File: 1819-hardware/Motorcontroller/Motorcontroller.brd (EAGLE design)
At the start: 44.8 x 54 mm, 36 parts, among them U1 MAX3485CSA, U3 PCA9306, U4 74HC1G04

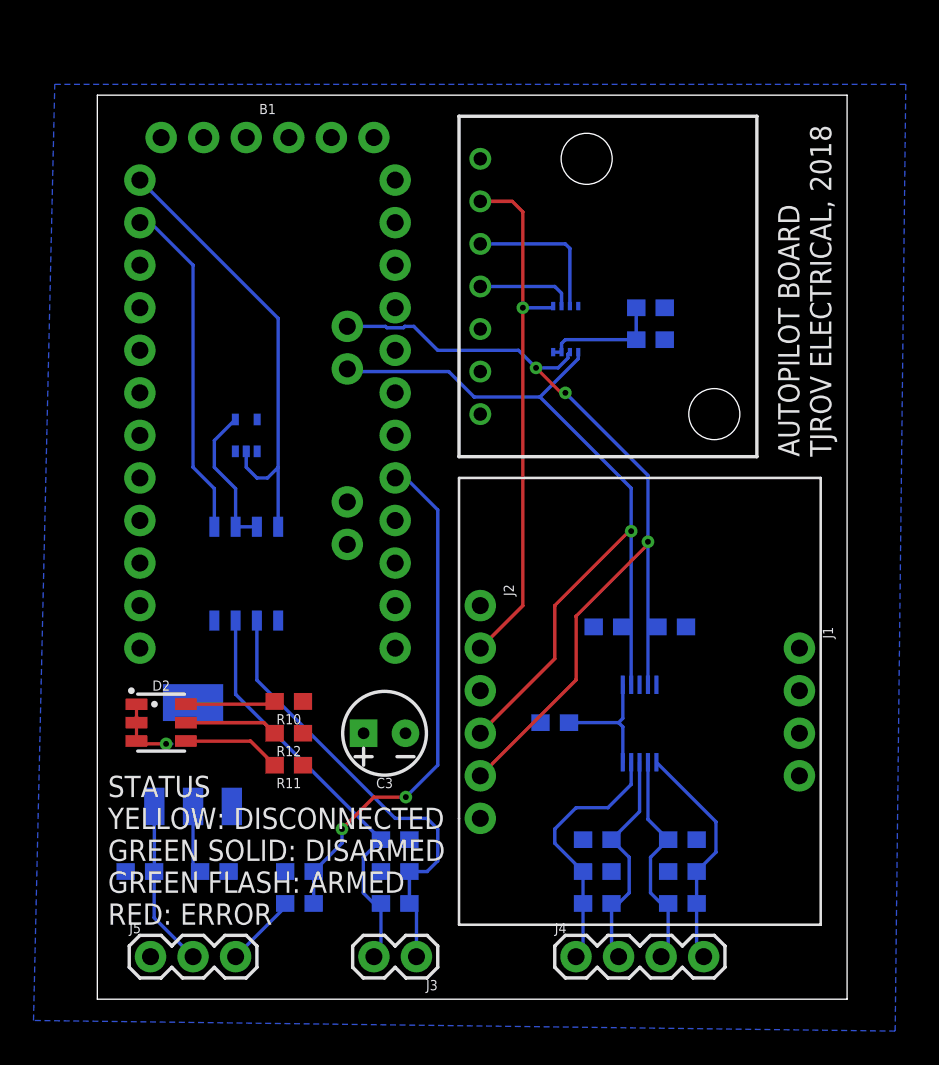
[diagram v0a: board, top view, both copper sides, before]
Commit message: started motorcontroller board files
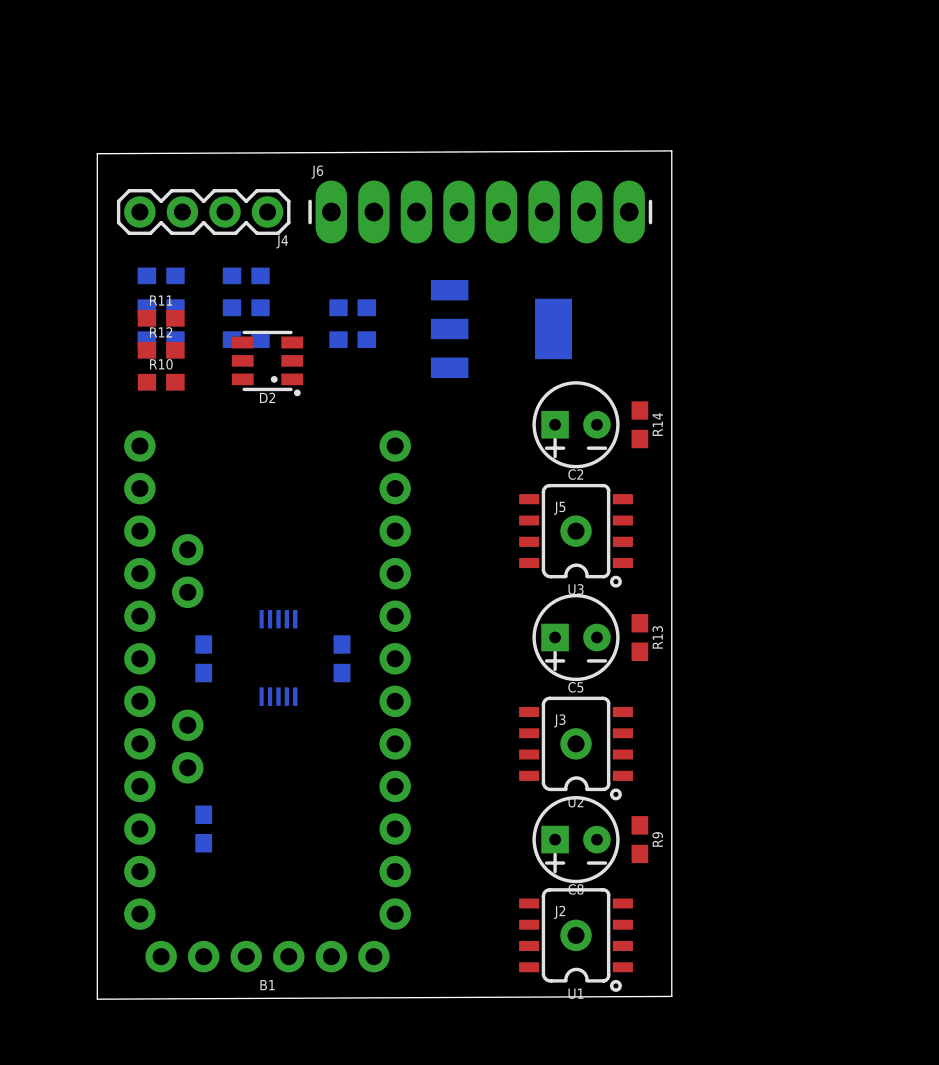
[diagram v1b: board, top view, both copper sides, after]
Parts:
- removed B2: Pressure Sensor, SparkFun-Boards:SPARKFUN_MS5803-14BA_BREAKOUT
- removed J1: (no value), SparkFun-Connectors:1X04_NO_SILK
- removed R15, R17: 4.7k, SparkFun-Resistors:0603
- removed R16: 100k, SparkFun-Resistors:0603
- removed U4: 74HC1G04, SparkFun-IC-Logic:SOT353
- added C8: 10uF, SparkFun-Capacitors:CPOL-RADIAL-2.5MM-5MM
- added J6: (no value), SparkFun-Connectors:1X08_LONGPADS
- added U2: GENERIC-SOIC8MSGEQ7N-FILTER, SparkFun-Retired:SO08
- C2, C5: value 0.1uF -> 10uF; device SparkFun-Capacitors:0603 -> SparkFun-Capacitors:CPOL-RADIAL-2.5MM-5MM
- C3: value 10uF -> 0.1uF; device SparkFun-Capacitors:CPOL-RADIAL-2.5MM-5MM -> SparkFun-Capacitors:0603
- J2: device SparkFun-Connectors:1X06_NO_SILK -> SparkFun-Connectors:1X01_NO_SILK
- J3: device SparkFun-Connectors:1X02 -> SparkFun-Connectors:1X01_NO_SILK
- J5: device SparkFun-Connectors:1X03 -> SparkFun-Connectors:1X01_NO_SILK
- R1: value 100 -> 4.7k
- R13: value 100k -> 47k
- R14: value 4.7k -> 47k
- R4: value 680 -> 4.7k
- R9: value 680 -> 47k
- U1: value MAX3485CSA -> GENERIC-SOIC8MSGEQ7N-FILTER; device SparkFun-IC-Comms:SO08 -> SparkFun-Retired:SO08
- U3: value PCA9306 -> GENERIC-SOIC8MSGEQ7N-FILTER; device SparkFun-IC-Comms:PSOP-8 -> SparkFun-Retired:SO08
- moved FRAME1 121.6 mm to (-80.0, 47.0)
- moved R3 48.7 mm to (3.81, 43.2), turned to 180 degrees
- moved J4 48.1 mm to (10.2, 47.0), turned to 180 degrees
- moved R6 45.8 mm to (3.81, 41.3), turned to 0 degrees
- moved R7 43.1 mm to (3.81, 39.4), turned to 0 degrees
- moved R2 42.9 mm to (8.89, 43.2), turned to 0 degrees
- moved R5 39.6 mm to (8.89, 41.3), turned to 180 degrees
- moved R8 36.5 mm to (8.89, 39.4), turned to 180 degrees
- moved C6 36.0 mm to (15.2, 41.3)
- moved J5 35.9 mm to (28.6, 27.9)
- moved C2 34.3 mm to (28.6, 34.3), flipped to the top
- moved U$1 31.4 mm to (24.1, 40.0), turned to 90 degrees
- moved U1 29.2 mm to (28.6, 3.81), flipped to the top, turned to 90 degrees
- moved R11 27.7 mm to (3.81, 40.6), turned to 0 degrees
- moved C1 25.8 mm to (15.2, 39.4)
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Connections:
- removed net 3V3: B2.3.3V, J2.2, U3.1
- removed net 485A: J3.1, R1.1, R4.2, U1.6
- removed net 485B: J3.2, R1.2, R9.1, U1.7
- removed net N$19: C5.1, R13.1, U3.7, U3.8
- removed net RESET: B1.13, B1.3
- removed net RX: B1.2, U1.1
- removed net SCL3V3: B2.SCL/SCLK, U3.2
- removed net SDA3V3: B2.SDA/SDI, U3.3
- removed net TX: B1.1, U1.4, U4.2
- removed net VOLTAGE_SENSOR: B1.17, R16.1, R17.2
- new net M1DIR1: J6.3
- new net M1DIR2: J6.4
- new net M1IN1: B1.6, U1.3
- new net M1IN2: B1.8, U1.2
- new net M1OUT1: U1.6
- new net M1OUT2: U1.8
- new net M2DIR1: J6.5
- new net M2DIR2: J6.6
- new net M2IN1: B1.9, U2.3
- new net M2IN2: B1.12, U2.2
- new net M2OUT1: U2.6
- new net M2OUT2: U2.8
- new net M3DIR1: J6.7
- new net M3DIR2: J6.8
- new net M3IN1: B1.13, U3.3
- new net M3IN2: B1.14, U3.2
- new net M3OUT1: U3.6
- new net M3OUT2: U3.8
- new net N$2: R14.2, U3.4
- new net N$7: R9.2, U1.4
- net 12V: no longer J5.2
- net BATT: now also C2.1, C5.1, C8.1, J6.2, U1.5, U2.5, U3.5; no longer J5.3, R16.2
- net BLUE: now also B1.16; no longer B1.14
- net GND: now also C8.2, J2.1, J3.1, J6.1, R13.1, R14.1, R9.1, U1.1, U1.7, U2.1, U2.7, U3.1, U3.7; no longer B2.GND, J2.3, R17.1, R4.1, U1.5, U3.4, U4.3
- net N$1: now also R13.2, U2.4; no longer U1.2, U1.3, U4.4
- net RED: now also B1.11; no longer B1.16
- net SCL: now also R1.1; no longer J2.5, R14.2, U3.6
- net SDA: now also R4.1; no longer J2.4, R15.2, U3.5
- net VCC: now also R1.2, R4.2; no longer C2.1, J2.1, R13.2, R14.1, R15.1, R9.2, U1.8, U4.5
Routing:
- net SCL: track 54.9 -> 0.00 mm, vias 3 -> 0
- net SDA: track 51.1 -> 0.00 mm, vias 1 -> 0
- net 3V3: track 31.7 -> 0.00 mm, vias 1 -> 0
- net VOLTAGE_SENSOR: track 31.0 -> 0.00 mm, vias 2 -> 0
- net TX: track 27.5 -> 0.00 mm
- net 485A: track 27.1 -> 0.00 mm
- net 485B: track 24.9 -> 0.00 mm
- net RX: track 20.4 -> 0.00 mm
- net SDA-: track 15.5 -> 0.00 mm
- net SCL-: track 13.7 -> 0.00 mm
- net SDA+: track 13.6 -> 0.00 mm
- net SCL+: track 13.4 -> 0.00 mm
- net VCC: track 11.9 -> 0.00 mm
- net 12V: track 9.93 -> 0.00 mm
- net SDA3V3: track 8.90 -> 0.00 mm
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- removed copper zone on layer 16, net GND
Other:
- board size 44.8 x 54 mm -> 34.3 x 50.6 mm
- board text removed: "AUTOPILOT BOARD TJROV ELECTRICAL, 2018"
- board text removed: "STATUS YELLOW: DISCONNECTED GREEN SOLID: DISARMED GREEN FLASH: ARMED RED: ERROR"
